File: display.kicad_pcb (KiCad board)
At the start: 2 copper layers, 128.9 x 78.1 mm, 42 parts, among them J8 Screw_Terminal_1x04, U1 LM317T, U2 LM317T

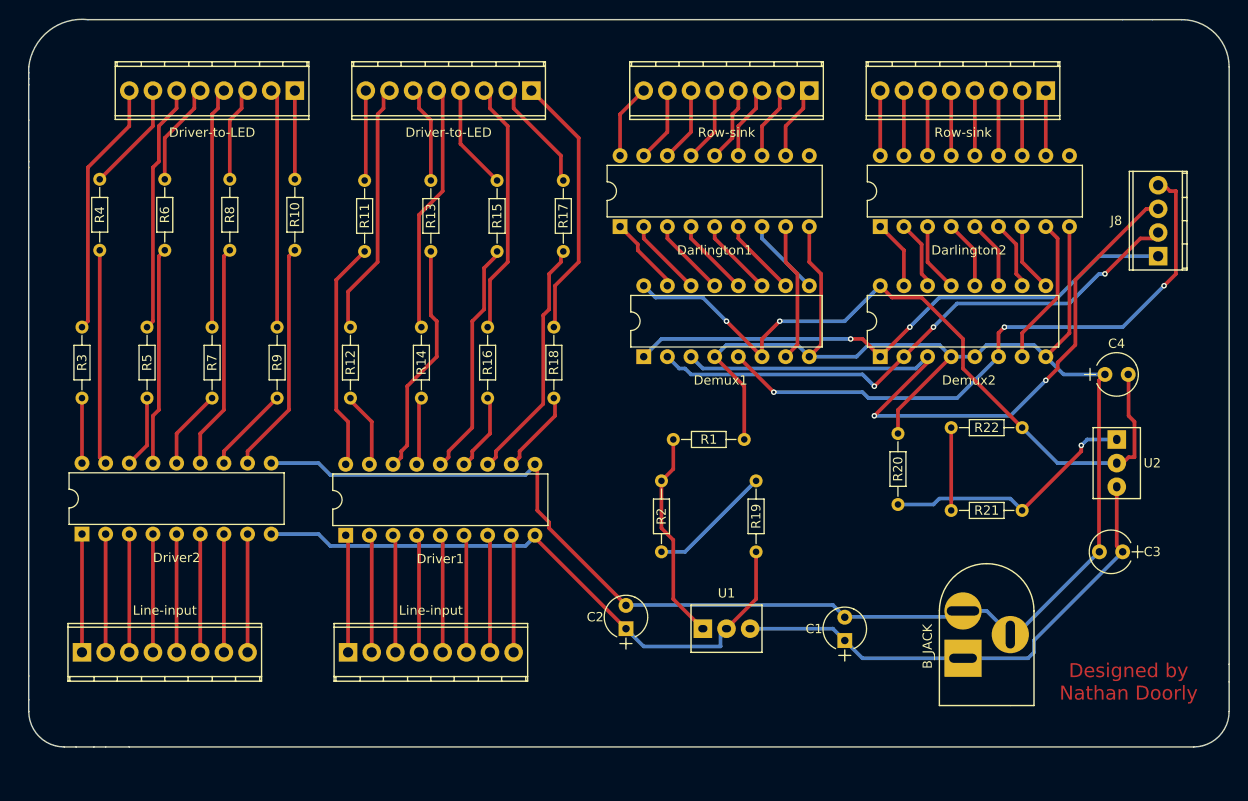
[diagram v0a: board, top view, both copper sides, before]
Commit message: Beth's updated copy pre-change
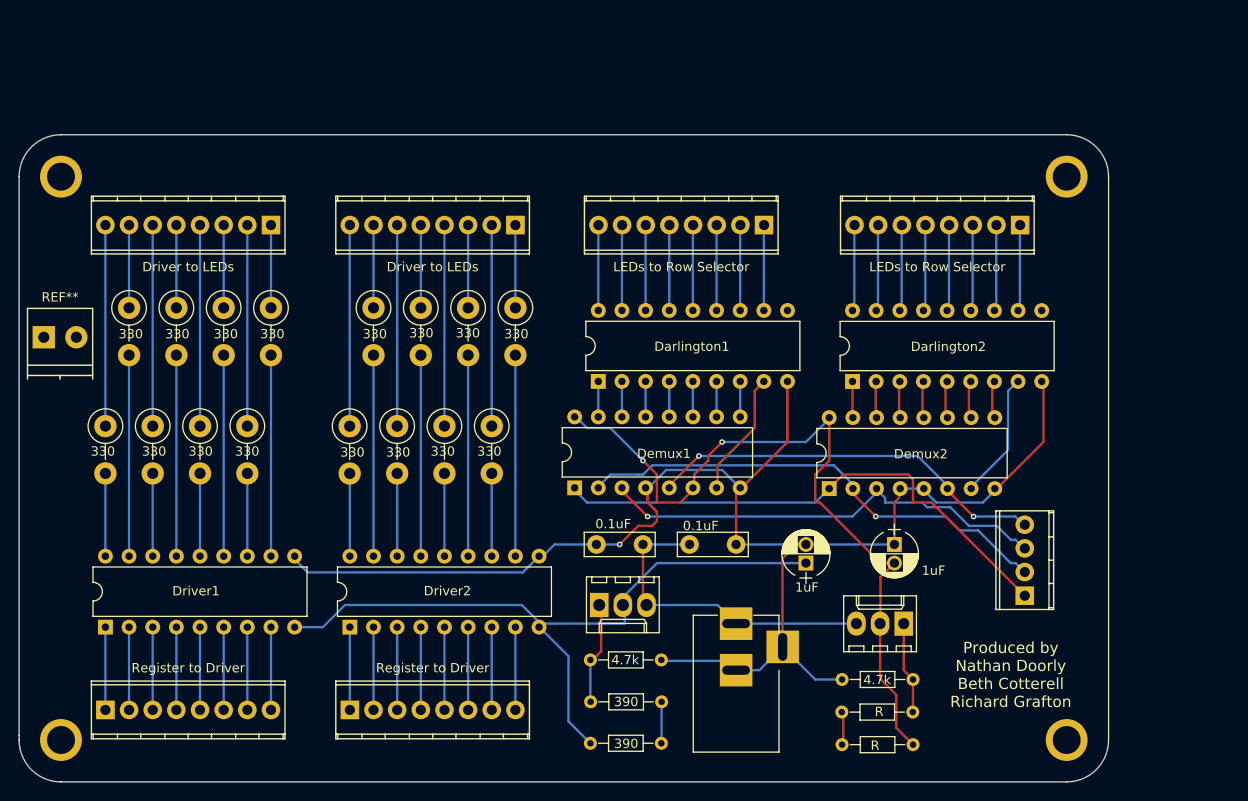
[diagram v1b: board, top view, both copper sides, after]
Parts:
- removed B_JACK: BARREL_JACK, new-lib:Barrel_Jack
- removed C1, C3: 0.1micF, Capacitors_THT:CP_Radial_Tantal_D4.5mm_P2.50mm
- removed C2, C4: 1micF, Capacitors_THT:CP_Radial_Tantal_D4.5mm_P2.50mm
- removed Driver-to-LED (x2), Line-input (x2), Row-sink (x2): Screw_Terminal_1x08, Connectors_Terminal_Blocks:TerminalBlock_Pheonix_MPT-2.54mm_8pol
- removed J8: Screw_Terminal_1x04, Connectors_Terminal_Blocks:TerminalBlock_Pheonix_MPT-2.54mm_4pol
- removed R1, R20: 4.7k, Resistors_THT:R_Axial_DIN0204_L3.6mm_D1.6mm_P7.62mm_Horizontal
- removed R10, R11, R12, R13, R14, R15, R16, R17, R18, R21, R22, R3, R4, R5, R6, R7, R8, R9: R, Resistors_THT:R_Axial_DIN0204_L3.6mm_D1.6mm_P7.62mm_Horizontal
- removed R19, R2: 390, Resistors_THT:R_Axial_DIN0204_L3.6mm_D1.6mm_P7.62mm_Horizontal
- removed U1, U2: LM317T, new-lib:LM317T
- added 0.1uF: , Capacitors_THT:C_Disc_D7.5mm_W2.5mm_P5.00mm, F.Cu at (132.0, 97.0)
- added 0.1uF: , Capacitors_THT:C_Disc_D7.5mm_W2.5mm_P5.00mm, F.Cu at (137.0, 97.0)
- added 1uF: , Capacitors_THT:CP_Radial_D5.0mm_P2.00mm, F.Cu at (159.0, 97.0)
- added 1uF: , Capacitors_THT:CP_Radial_D5.0mm_P2.00mm, F.Cu at (149.5, 99.0)
- added 330: R, Resistors_THT:R_Axial_DIN0411_L9.9mm_D3.6mm_P5.08mm_Vertical, F.Cu at (105.6, 84.3)
- added 330: R, Resistors_THT:R_Axial_DIN0411_L9.9mm_D3.6mm_P5.08mm_Vertical, F.Cu at (76.8, 71.6)
- added 330: R, Resistors_THT:R_Axial_DIN0411_L9.9mm_D3.6mm_P5.08mm_Vertical, F.Cu at (79.3, 84.3)
- added 330: R, Resistors_THT:R_Axial_DIN0411_L9.9mm_D3.6mm_P5.08mm_Vertical, F.Cu at (81.9, 71.6)
- added 330: R, Resistors_THT:R_Axial_DIN0411_L9.9mm_D3.6mm_P5.08mm_Vertical, F.Cu at (84.4, 84.3)
- added 330: R, Resistors_THT:R_Axial_DIN0411_L9.9mm_D3.6mm_P5.08mm_Vertical, F.Cu at (87.0, 71.6)
- added 330: R, Resistors_THT:R_Axial_DIN0411_L9.9mm_D3.6mm_P5.08mm_Vertical, F.Cu at (89.5, 84.3)
- added 330: R, Resistors_THT:R_Axial_DIN0411_L9.9mm_D3.6mm_P5.08mm_Vertical, F.Cu at (92.0, 71.6)
- added 330: R, Resistors_THT:R_Axial_DIN0411_L9.9mm_D3.6mm_P5.08mm_Vertical, F.Cu at (100.5, 84.3)
- added 330: R, Resistors_THT:R_Axial_DIN0411_L9.9mm_D3.6mm_P5.08mm_Vertical, F.Cu at (103.1, 71.6)
- added 330: R, Resistors_THT:R_Axial_DIN0411_L9.9mm_D3.6mm_P5.08mm_Vertical, F.Cu at (108.1, 71.6)
- added 330: R, Resistors_THT:R_Axial_DIN0411_L9.9mm_D3.6mm_P5.08mm_Vertical, F.Cu at (110.7, 84.3)
- added 330: R, Resistors_THT:R_Axial_DIN0411_L9.9mm_D3.6mm_P5.08mm_Vertical, F.Cu at (113.2, 71.6)
- added 330: R, Resistors_THT:R_Axial_DIN0411_L9.9mm_D3.6mm_P5.08mm_Vertical, F.Cu at (115.8, 84.3)
- added 330: R, Resistors_THT:R_Axial_DIN0411_L9.9mm_D3.6mm_P5.08mm_Vertical, F.Cu at (118.3, 71.6)
- added 330: R, Resistors_THT:R_Axial_DIN0411_L9.9mm_D3.6mm_P5.08mm_Vertical, F.Cu at (74.3, 84.3)
- added 390: , Resistors_THT:R_Axial_DIN0204_L3.6mm_D1.6mm_P7.62mm_Horizontal, F.Cu at (134.0, 113.9)
- added 390: , Resistors_THT:R_Axial_DIN0204_L3.6mm_D1.6mm_P7.62mm_Horizontal, F.Cu at (126.3, 118.3)
- added 4.7k: , Resistors_THT:R_Axial_DIN0204_L3.6mm_D1.6mm_P7.62mm_Horizontal, F.Cu at (126.3, 109.4)
- added 4.7k: , Resistors_THT:R_Axial_DIN0204_L3.6mm_D1.6mm_P7.62mm_Horizontal, F.Cu at (161.0, 111.5)
- added ?: Screw_Terminal_1x04, Connectors_Terminal_Blocks:TerminalBlock_Pheonix_MPT-2.54mm_4pol, F.Cu at (173.0, 102.5)
- added ?: LM317T, Connectors_Molex:Molex_KK-6410-03_03x2.54mm_Straight, F.Cu at (127.3, 103.5)
- added ?: LM317T, Connectors_Molex:Molex_KK-6410-03_03x2.54mm_Straight, F.Cu at (160.0, 105.5)
- added ?: BARREL_JACK, Connectors:BARREL_JACK, F.Cu at (142.0, 105.5)
- added ?: 3mm drill, Wire_Pads:SolderWirePad_single_2mmDrill, F.Cu at (69.5, 57.5)
- added ?: 3mm drill hole, Wire_Pads:SolderWirePad_single_2mmDrill, F.Cu at (177.5, 57.5)
- added ?: 3mm drill hole, Wire_Pads:SolderWirePad_single_2mmDrill, F.Cu at (177.5, 118.0)
- added ?: 3mm drill hole, Wire_Pads:SolderWirePad_single_2mmDrill, F.Cu at (69.5, 118.0)
- added Driver to LEDs: Screw_Terminal_1x08, Connectors_Terminal_Blocks:TerminalBlock_Pheonix_MPT-2.54mm_8pol, F.Cu at (118.3, 62.7)
- added Driver to LEDs: Screw_Terminal_1x08, Connectors_Terminal_Blocks:TerminalBlock_Pheonix_MPT-2.54mm_8pol, F.Cu at (92.0, 62.7)
- added LEDs to Row Selector: Screw_Terminal_1x08, Connectors_Terminal_Blocks:TerminalBlock_Pheonix_MPT-2.54mm_8pol, F.Cu at (172.5, 62.7)
- added LEDs to Row Selector: Screw_Terminal_1x08, Connectors_Terminal_Blocks:TerminalBlock_Pheonix_MPT-2.54mm_8pol, F.Cu at (145.0, 62.7)
- added R: , Resistors_THT:R_Axial_DIN0204_L3.6mm_D1.6mm_P7.62mm_Horizontal, F.Cu at (153.3, 115.0)
- added R: , Resistors_THT:R_Axial_DIN0204_L3.6mm_D1.6mm_P7.62mm_Horizontal, F.Cu at (161.0, 118.5)
- added REF**: TerminalBlock_Pheonix_PT-3.5mm_2pol, Connectors_Terminal_Blocks:TerminalBlock_Pheonix_PT-3.5mm_2pol, F.Cu at (67.7, 74.8)
- added Register to Driver: Screw_Terminal_1x08, Connectors_Terminal_Blocks:TerminalBlock_Pheonix_MPT-2.54mm_8pol, F.Cu at (100.5, 114.8)
- added Register to Driver: Screw_Terminal_1x08, Connectors_Terminal_Blocks:TerminalBlock_Pheonix_MPT-2.54mm_8pol, F.Cu at (74.3, 114.8)
- moved Driver2 30.5 mm to (100.5, 105.9)
- moved Driver1 27.6 mm to (74.3, 105.9)
- moved Darlington2 16.9 mm to (154.5, 79.5)
- moved Darlington1 16.8 mm to (127.2, 79.5)
- moved Demux1 15.9 mm to (124.7, 90.9)
- moved Demux2 15.2 mm to (152.0, 91.0)
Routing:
- net GND: track 222.0 -> 166.8 mm, vias 0 -> 1
- net Net-(Demux1-Pad3): track 79.3 -> 49.8 mm, vias 2 -> 1
- net Net-(Demux1-Pad5): track 66.9 -> 43.9 mm, vias 3 -> 2
- net Net-(J5-Pad1): track 28.7 -> 8.89 mm
- net Net-(C1-Pad1): track 54.0 -> 35.0 mm
- net Net-(J5-Pad7): track 27.5 -> 8.89 mm
- net Net-(J5-Pad3): track 27.5 -> 8.89 mm
- net Net-(J5-Pad5): track 27.0 -> 8.89 mm
- net Net-(R20-Pad1): track 27.8 -> 10.0 mm, vias 1 -> 0
- net Net-(Driver1-Pad12): track 26.6 -> 8.89 mm
- net Net-(Driver1-Pad14): track 25.7 -> 8.89 mm
- net Net-(Driver1-Pad16): track 25.1 -> 8.89 mm
- net Net-(Driver1-Pad18): track 24.8 -> 8.89 mm
- net Net-(Driver1-Pad15): track 7.52 -> 21.6 mm
- net Net-(Driver1-Pad13): track 8.58 -> 21.6 mm
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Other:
- board size 128.9 x 78.1 mm -> 117 x 69.5 mm
- rule pad_to_mask_clearance: 0.2 -> 0
- board text added: "Produced by Nathan Doorly Beth Cotterell Richard Grafton"
- board text removed: "Designed by Nathan Doorly"
